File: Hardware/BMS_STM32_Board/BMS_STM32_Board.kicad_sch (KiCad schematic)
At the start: 21 parts, among them J1 Conn_01x05, J2 Conn_01x02, J3 Conn_01x04, Q1 Q_PMOS_GSD, U1 STM32F103C8Tx, U2 INA180A1, Y1 8MHz

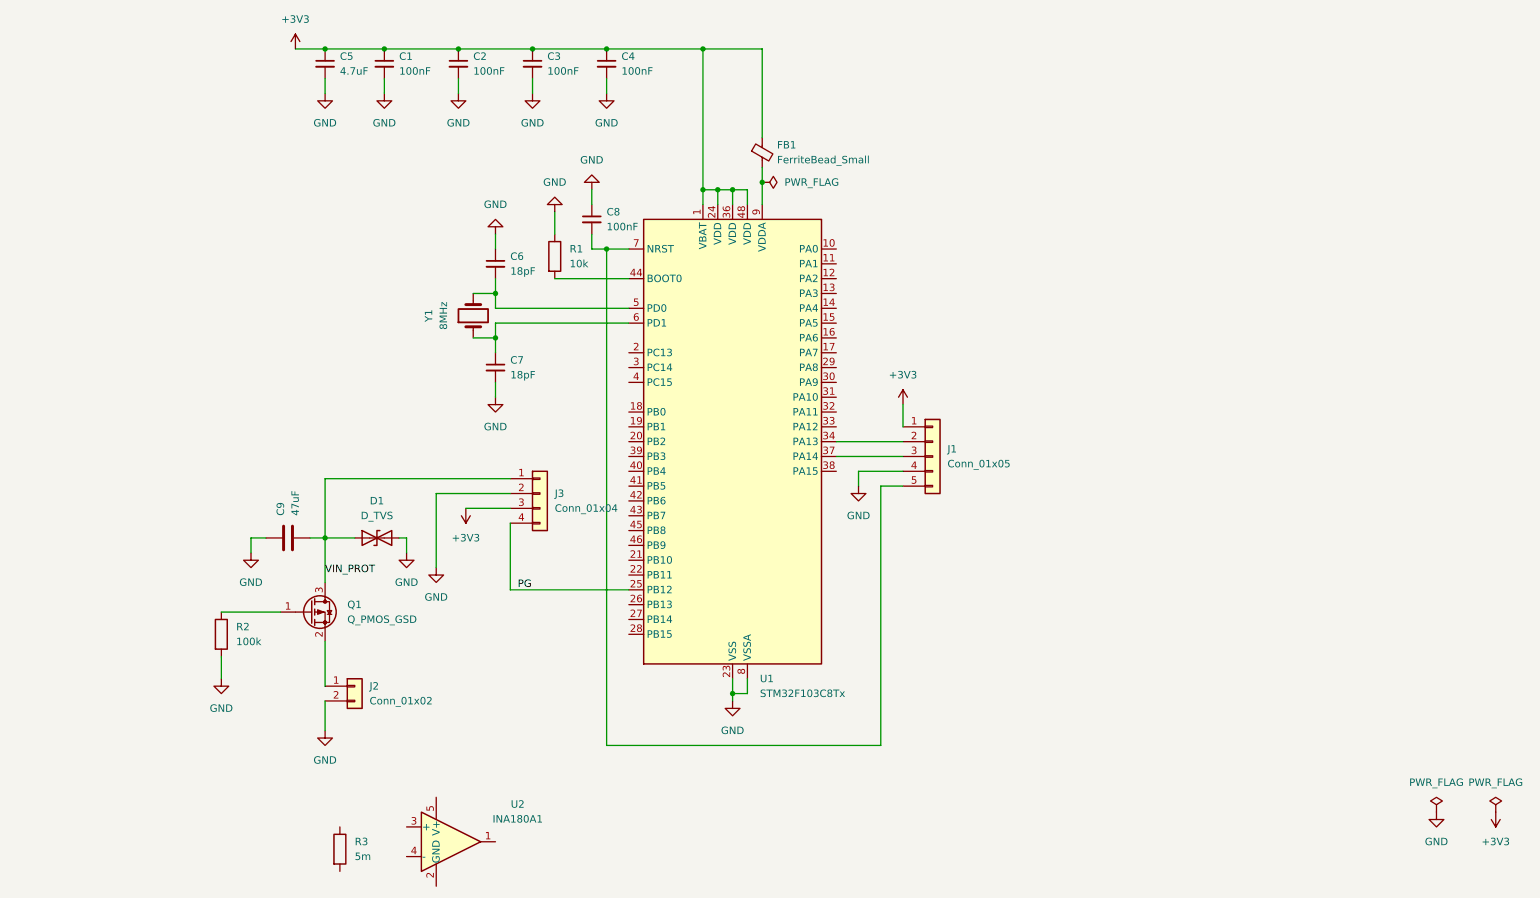
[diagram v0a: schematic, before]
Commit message: current sense
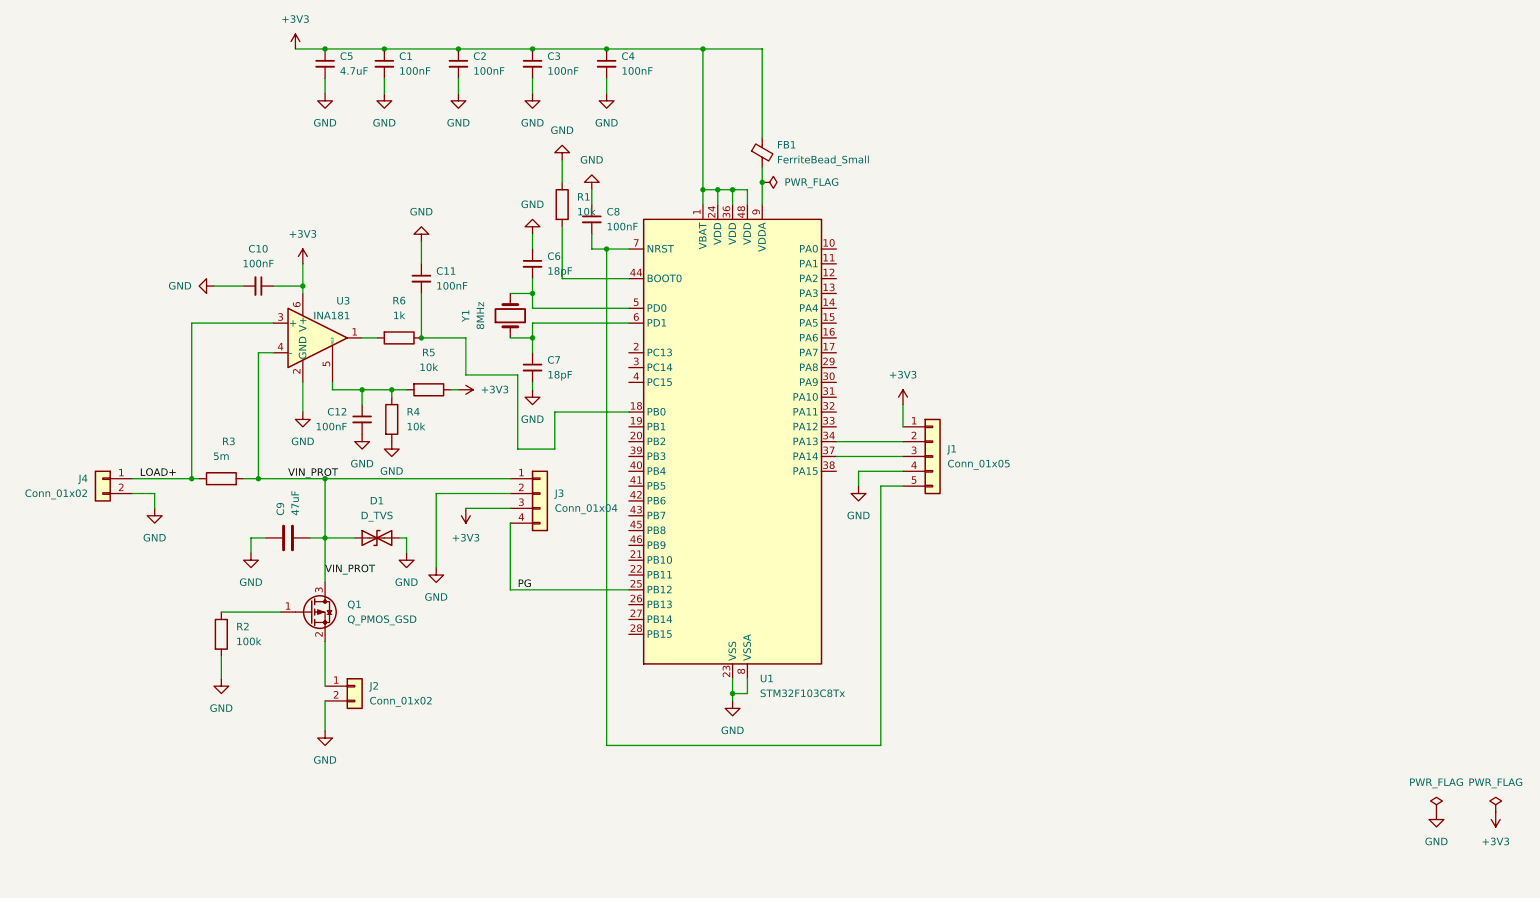
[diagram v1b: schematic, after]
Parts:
- removed U2: INA180A1, Package_TO_SOT_SMD:SOT-23-5, symbol Amplifier_Current:INA180A1
- added C10, C11, C12: 100nF, symbol Device:C_Small
- added J4: Conn_01x02, symbol Connector_Generic:Conn_01x02
- added R4, R5: 10k, symbol Device:R
- added R6: 1k, symbol Device:R
- added U3: INA181, Package_TO_SOT_SMD:SOT-23-6, symbol Amplifier_Current:INA181
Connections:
- net +3V3: now also C10.1, R5.1, U3.6 (V+)
- net GND: now also C10.2, C11.1, C12.2, J4.2 (Pin_2), R4.2, U3.2 (GND)
- net VIN_PROT: now also R3.2, U3.4 (-)
- net LOAD+: now reaches R3.1
- net LOAD+: now also J4.1 (Pin_1), U3.3 (+)
- net at U1.18 (PB0): now also C11.2, R6.1
- new net: C12.1, R4.1, R5.2, U3.5 (REF)
- new net: R6.2, U3.1
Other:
- moved on the sheet: C6, C7, R1, R3, Y1
